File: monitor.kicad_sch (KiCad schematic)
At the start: 44 parts, among them J1 Conn_01x01_Socket, J2 Conn_01x01_Socket, J3 Conn_01x01_Socket, J4 Conn_01x01_Socket, J5 Conn_01x01_Socket, J6 Conn_01x01_Socket, U704 OPA2197D, U76 OPA2189DGK, U77 OPA2388DGK, U78 OPA2189DGK

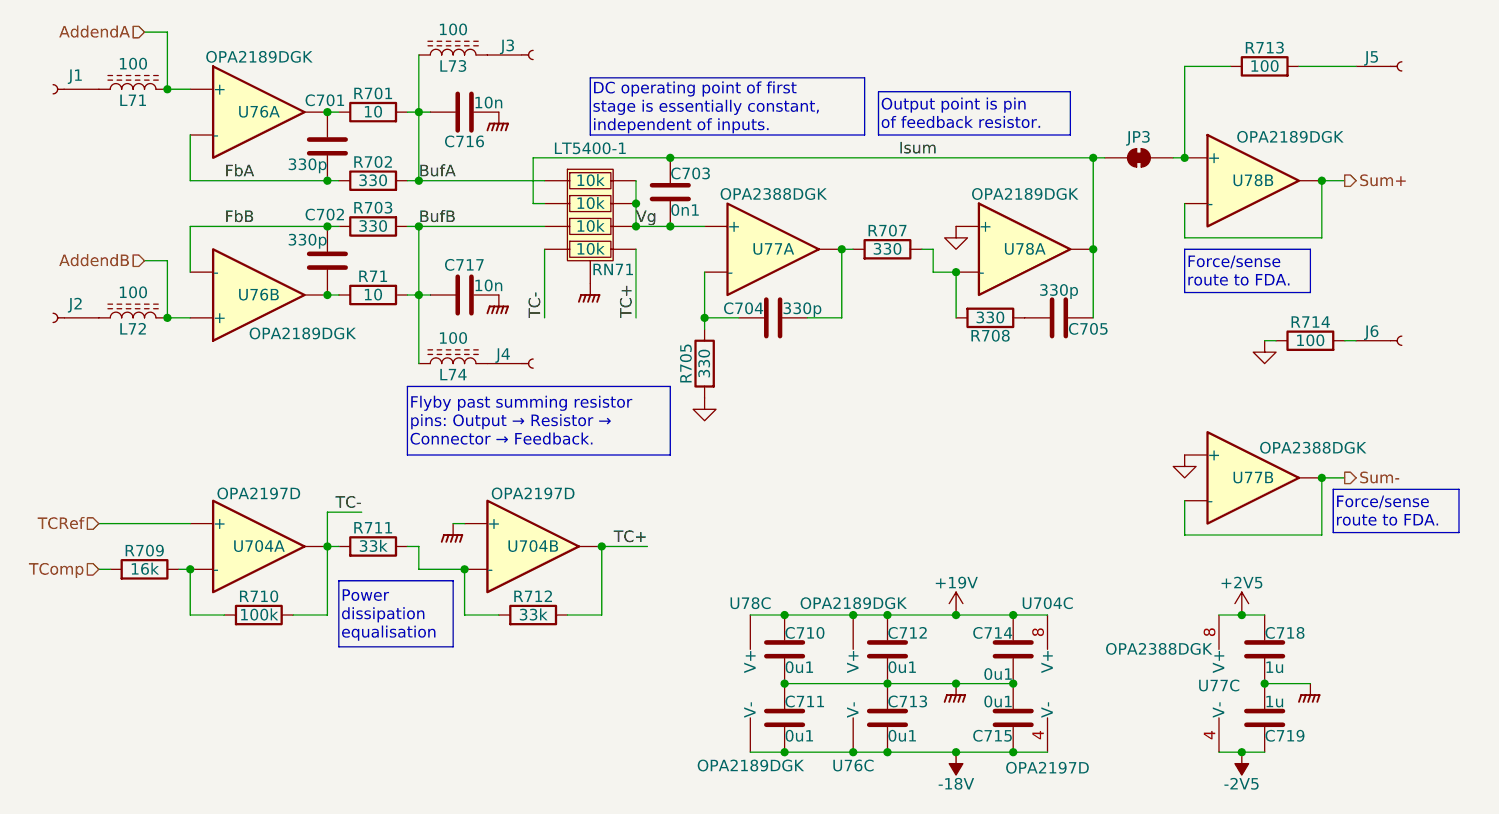
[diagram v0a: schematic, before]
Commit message: Progress checkin.  About to redo FDA feedback again.
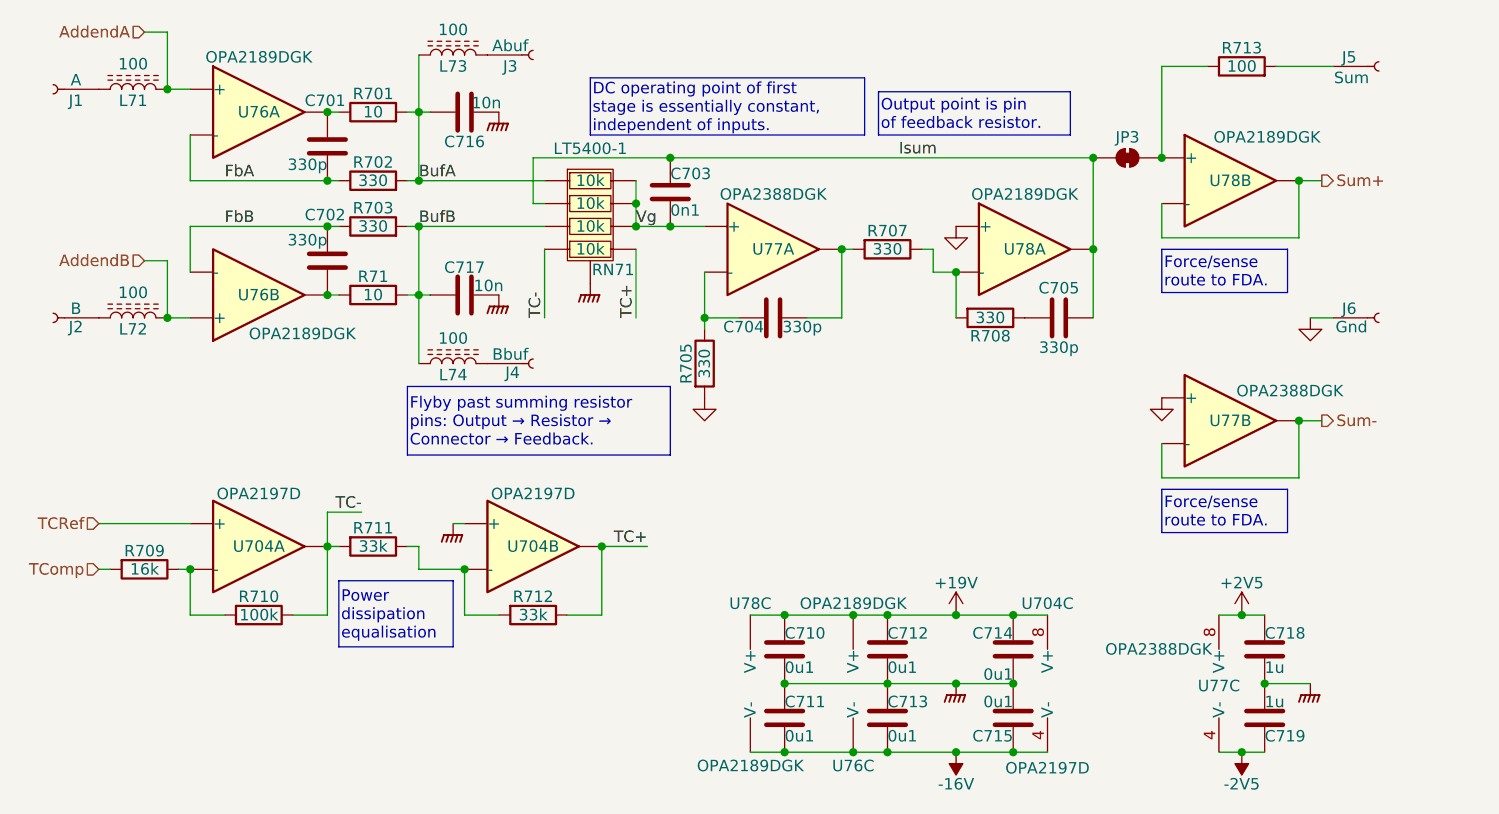
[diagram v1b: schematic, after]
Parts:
- removed R714: 100, Resistor_SMD:R_0402_1005Metric, symbol Device:R
- J1: value Conn_01x01_Socket -> A
- J2: value Conn_01x01_Socket -> B
- J3: value Conn_01x01_Socket -> Abuf
- J4: value Conn_01x01_Socket -> Bbuf
- J5: value Conn_01x01_Socket -> Sum
- J6: value Conn_01x01_Socket -> Gnd
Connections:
- net GND: now also J6.1 (Pin_1)
- net -18V renamed -16V
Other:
- moved on the sheet: J5, J6, JP3, R713, U77B, U78B
